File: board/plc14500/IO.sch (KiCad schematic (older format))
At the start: 70 parts, among them U1 74HC14, U11 74HC14, U2 4051, U3 74HC14, U4 NE555, U5 4099, U6 Arduino Nano

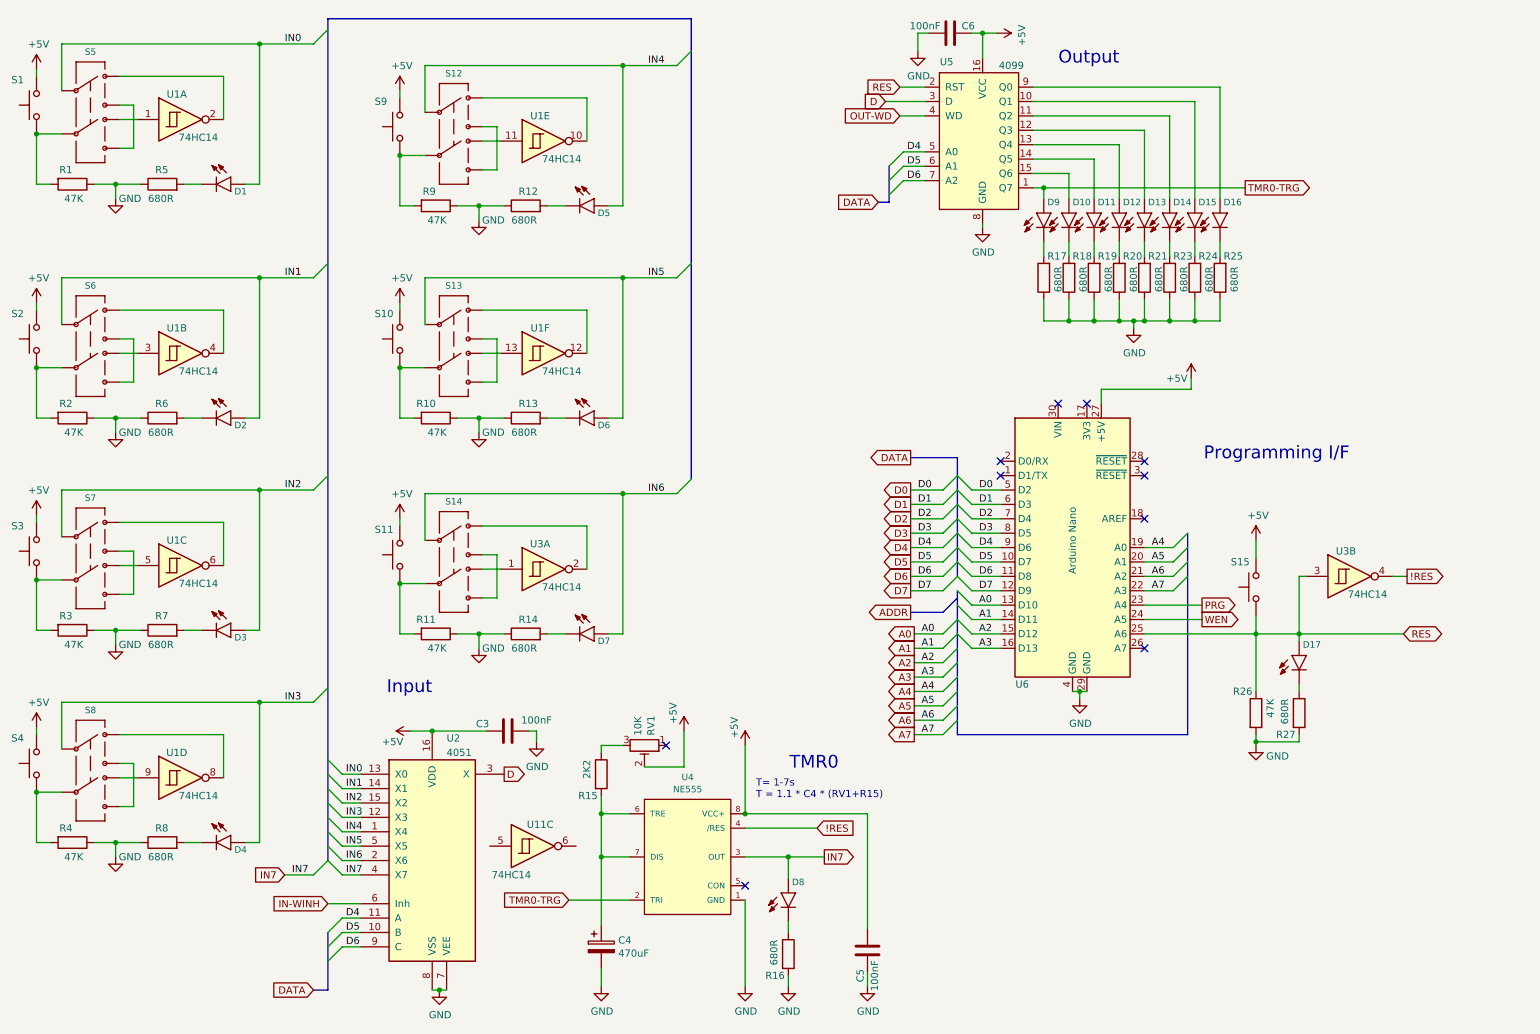
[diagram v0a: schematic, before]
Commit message: Rev_b board
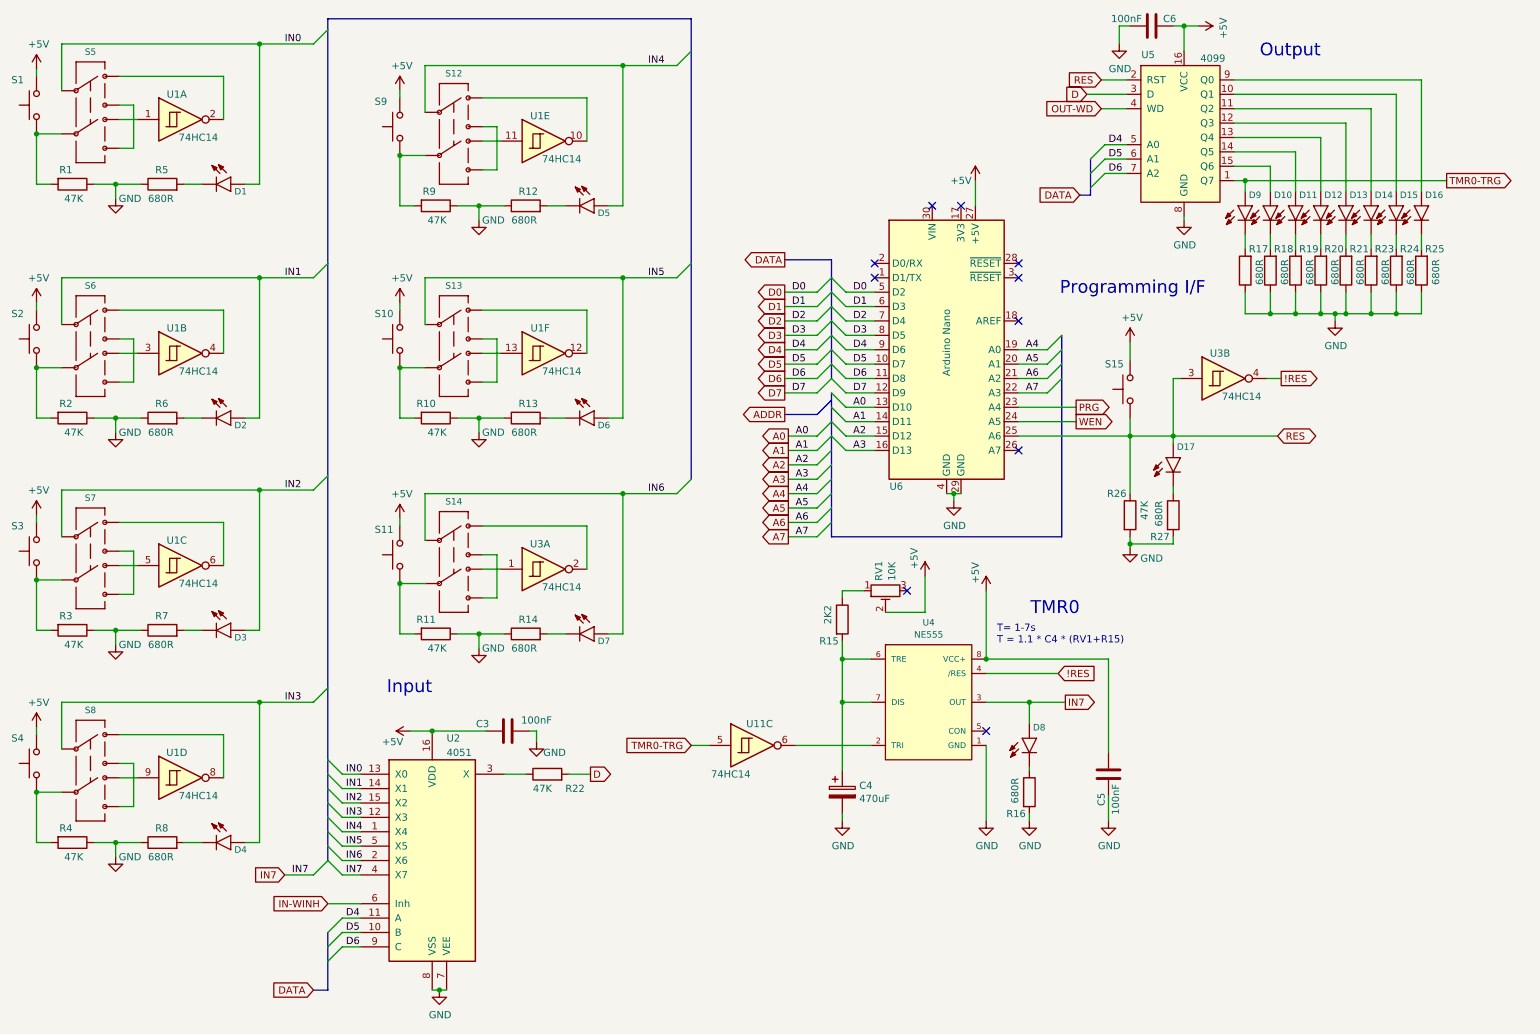
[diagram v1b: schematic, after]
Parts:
- added R22: 47K, Resistor_THT:R_Axial_DIN0204_L3.6mm_D1.6mm_P7.62mm_Horizontal, symbol Device:R
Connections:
- net D: now also R22.2; no longer U2.3 (X)
- net TMR0-TRG: now also U11.5; no longer U4.2 (TRI)
- net at U11.6: now also U4.2 (TRI)
- net at R15.1: now also RV1.1; no longer RV1.3
- new net: R22.1, U2.3 (X)
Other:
- moved on the sheet: C4, C5, C6, D10, D11, D12, D13, D14, D15, D16, D17, D8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
